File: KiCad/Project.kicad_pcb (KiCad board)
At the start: 2 copper layers, 0 parts

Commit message: Updated the schematics and started with the PCB
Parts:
- added C1, C2: 22pF, Capacitors_ThroughHole:C_Disc_D3_P2.5, F.Cu at (148.5, 105.0)
- added C3, C5: 0.1uF, Capacitors_ThroughHole:C_Disc_D3_P2.5, F.Cu at (148.5, 105.0)
- added C4, C6: 1uF, Capacitors_ThroughHole:C_Radial_D5_L6_P2.5, F.Cu at (148.5, 105.0)
- added D1, D11, D12, D13, D14, D15, D16, D2, D5, D6, D7, D8: LED, Wire_Connections_Bridges:WireConnection_1.50mmDrill, F.Cu at (148.5, 105.0)
- added D10, D3, D4, D9: IR_Recieve, Wire_Connections_Bridges:WireConnection_1.50mmDrill, F.Cu at (148.5, 105.0)
- added DS1: I2C_LCD16X2, Pin_Headers:Pin_Header_Straight_2x03_Pitch2.00mm, F.Cu at (148.5, 105.0)
- added IC1: ATMEGA328-P, Housings_DIP:DIP-28_W7.62mm, F.Cu at (146.1, 104.1)
- added IC2, IC3: ATTINY85-P, Housings_DIP:DIP-8_W7.62mm, F.Cu at (148.5, 105.0)
- added IC4: ATMEGA8-P, Housings_DIP:DIP-28_W7.62mm, F.Cu at (148.5, 105.0)
- added M1, M2: Motor, Wire_Connections_Bridges:WireConnection_1.50mmDrill, F.Cu at (148.5, 105.0)
- added P1: CONN_02X03, Pin_Headers:Pin_Header_Angled_2x03, F.Cu at (148.5, 105.0)
- added Q2, Q3, Q4: Q_NPN_BCE, TO_SOT_Packages_THT:TO-92_Inline_Narrow_Oval, F.Cu at (148.5, 105.0)
- added Q5: NPN, TO_SOT_Packages_THT:TO-92_Inline_Narrow_Oval, F.Cu at (148.5, 105.0)
- added R1: 1k, Resistors_ThroughHole:Resistor_Vertical_RM5mm, F.Cu at (148.5, 105.0)
- added R10, R11, R16, R17: 100, Resistors_ThroughHole:Resistor_Vertical_RM5mm, F.Cu at (148.5, 105.0)
- added R12, R13, R14, R15, R18, R19, R31, R37, R8, R9: 22, Resistors_ThroughHole:Resistor_Vertical_RM5mm, F.Cu at (148.5, 105.0)
- added R2: 10k, Resistors_ThroughHole:Resistor_Vertical_RM5mm, F.Cu at (148.5, 105.0)
- added R20, R21, R29, R30, R5: 1K, Resistors_ThroughHole:Resistor_Vertical_RM5mm, F.Cu at (148.5, 105.0)
- added R22, R6: 330, Resistors_ThroughHole:Resistor_Vertical_RM5mm, F.Cu at (148.5, 105.0)
- added R3: Photores, Wire_Connections_Bridges:WireConnection_1.50mmDrill, F.Cu at (148.5, 105.0)
- added R32, R33: 10, Resistors_ThroughHole:Resistor_Vertical_RM5mm, F.Cu at (148.5, 105.0)
- added R34, R35, R36: R, Resistors_ThroughHole:Resistor_Vertical_RM5mm, F.Cu at (148.5, 105.0)
- added R38, R39: 56, Resistors_ThroughHole:Resistor_Vertical_RM5mm, F.Cu at (148.5, 105.0)
- added R7: 470, Resistors_ThroughHole:Resistor_Vertical_RM5mm, F.Cu at (148.5, 105.0)
- added SW1: Reverse, Wire_Connections_Bridges:WireConnection_1.50mmDrill, F.Cu at (148.5, 105.0)
- added SW2: Start, Wire_Connections_Bridges:WireConnection_1.50mmDrill, F.Cu at (148.5, 105.0)
- added SW3: Lights, Wire_Connections_Bridges:WireConnection_1.50mmDrill, F.Cu at (148.5, 105.0)
- added SW4: SW_PUSH, Wire_Connections_Bridges:WireConnection_1.50mmDrill, F.Cu at (148.5, 105.0)
- added U1: BlueSmirf, Pin_Headers:Pin_Header_Straight_1x06, F.Cu at (148.5, 105.0)
- added U2, U3: LM317, TO_SOT_Packages_THT:TO-220_Neutral123_Vertical, F.Cu at (148.5, 105.0)
- added U5: Linkura, Wire_Connections_Bridges:WireConnection_1.50mmDrill, F.Cu at (148.5, 105.0)
- added U6: SN754410NE, Housings_DIP:DIP-16_W7.62mm_LongPads, F.Cu at (148.5, 105.0)
- added Y1: Crystal, Crystals:Crystal_HC52-U_Vertical, F.Cu at (148.5, 105.0)
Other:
- board outline added: 170.2 x 123.2 mm

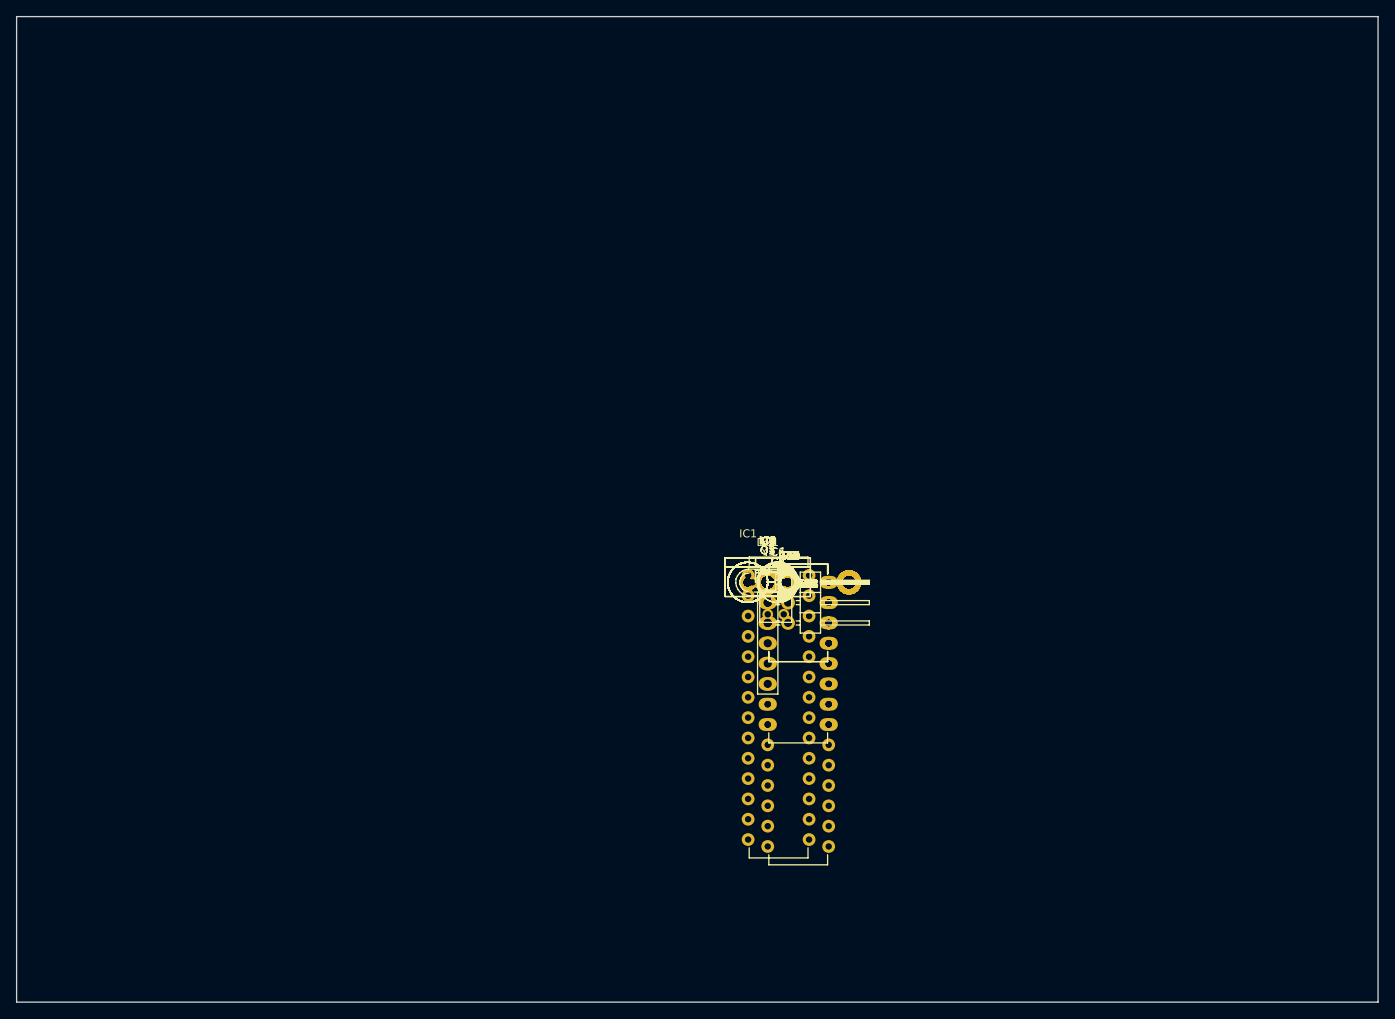
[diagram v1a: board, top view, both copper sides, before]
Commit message: Started with the PCB
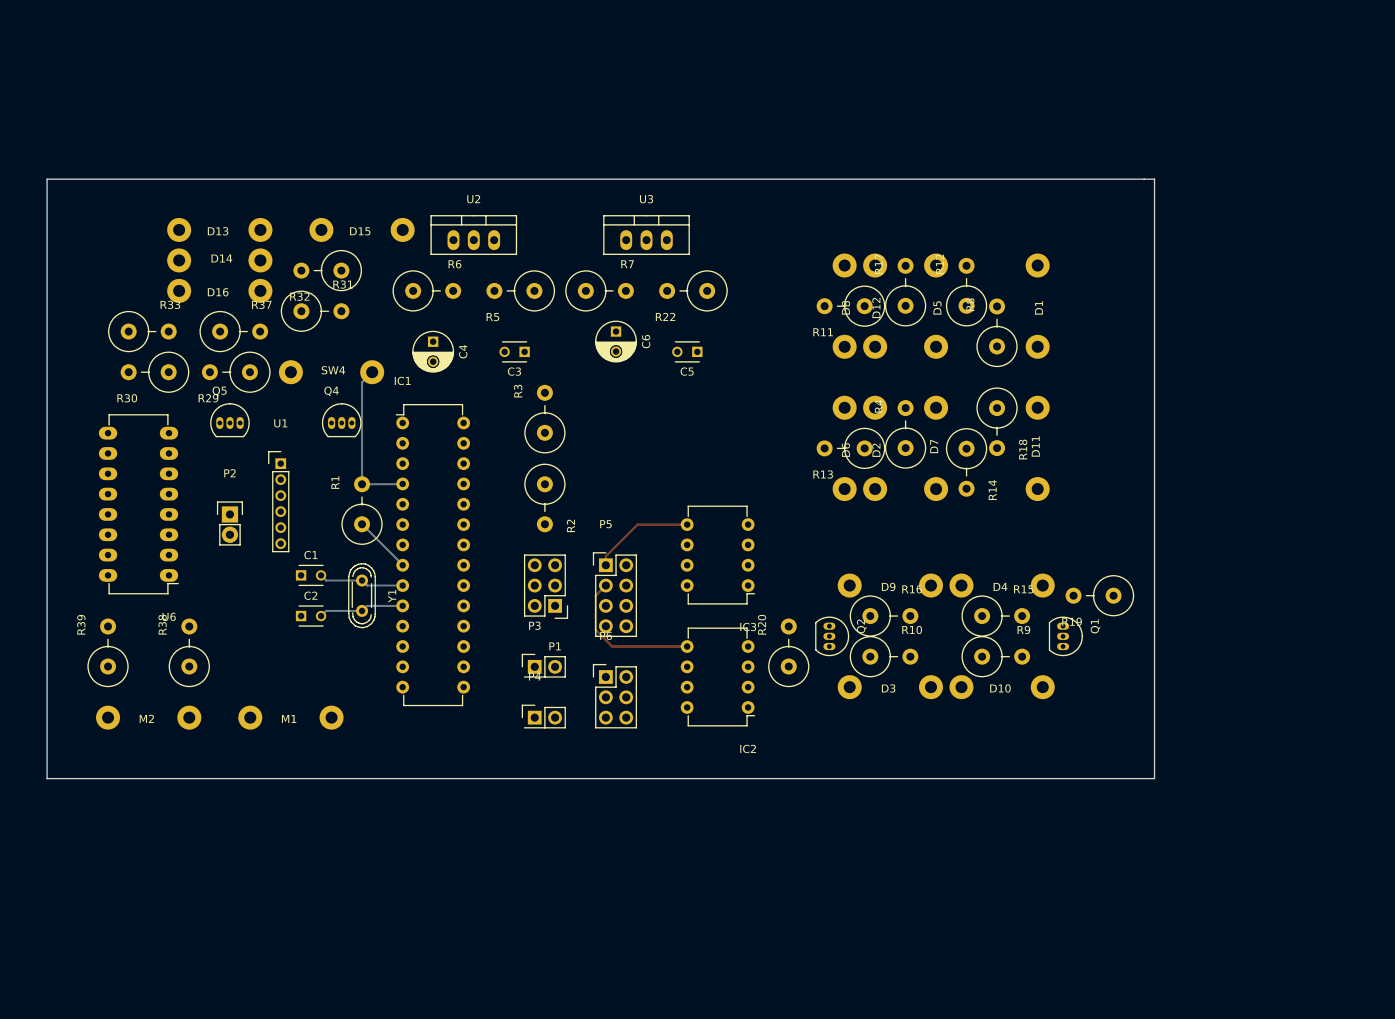
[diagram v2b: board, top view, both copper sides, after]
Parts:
- removed DS1: I2C_LCD16X2, Pin_Headers:Pin_Header_Straight_2x03_Pitch2.00mm
- removed IC4: ATMEGA8-P, Housings_DIP:DIP-28_W7.62mm
- removed Q3: Q_NPN_BCE, TO_SOT_Packages_THT:TO-92_Inline_Narrow_Oval
- removed R21: 1K, Resistors_ThroughHole:Resistor_Vertical_RM5mm
- removed R34, R35, R36: R, Resistors_ThroughHole:Resistor_Vertical_RM5mm
- removed SW1: Reverse, Wire_Connections_Bridges:WireConnection_1.50mmDrill
- removed SW2: Start, Wire_Connections_Bridges:WireConnection_1.50mmDrill
- removed SW3: Lights, Wire_Connections_Bridges:WireConnection_1.50mmDrill
- removed U5: Linkura, Wire_Connections_Bridges:WireConnection_1.50mmDrill
- added P2: CONN_01X02, Pin_Headers:Pin_Header_Straight_1x02, F.Cu at (81.3, 96.5)
- added P3: CONN_01X02, Pin_Headers:Pin_Header_Straight_2x01, F.Cu at (119.4, 115.6)
- added P4: CONN_01X02, Pin_Headers:Pin_Header_Straight_2x01, F.Cu at (119.4, 121.9)
- added P5: CONN_02X04, Pin_Headers:Pin_Header_Straight_2x04, F.Cu at (128.3, 102.9)
- added P6: CONN_02X03, Pin_Headers:Pin_Header_Straight_2x03, F.Cu at (128.3, 116.8)
- added Q1: Q_NPN_BCE, TO_SOT_Packages_THT:TO-92_Inline_Narrow_Oval, F.Cu at (185.4, 110.5)
- added R4: 22, Resistors_ThroughHole:Resistor_Vertical_RM5mm, F.Cu at (165.7, 85.7)
- P1: footprint Pin_Headers:Pin_Header_Angled_2x03 -> Pin_Headers:Pin_Header_Straight_2x03
- R11, R17: value 100 -> 22
- R15, R9: value 22 -> 100
- R19: value 22 -> 1K
- R3: footprint Wire_Connections_Bridges:WireConnection_1.50mmDrill -> Resistors_ThroughHole:Resistor_Vertical_RM5mm
- U1: footprint Pin_Headers:Pin_Header_Straight_1x06 -> Pin_Headers:Pin_Header_Straight_1x06_Pitch2.00mm
- moved D13 85.7 mm to (74.9, 61.0)
- moved M2 84.2 mm to (66.0, 121.9)
- moved R33 83.5 mm to (71.1, 73.7)
- moved R39 82.9 mm to (66.0, 113.0), turned to 90 degrees
- moved D16 82.1 mm to (74.9, 68.6)
- moved R30 81.7 mm to (71.1, 78.7), turned to 180 degrees
- moved D14 75.1 mm to (85.1, 64.8), turned to 180 degrees
- moved U6 74.8 mm to (73.7, 104.1), turned to 180 degrees
- moved R37 73.0 mm to (82.5, 73.7)
- moved R38 72.7 mm to (76.2, 113.0), turned to 90 degrees
- moved R29 72.2 mm to (81.3, 78.7), turned to 180 degrees
- moved Q5 71.3 mm to (80.0, 85.1)
- moved D15 71.1 mm to (92.7, 61.0)
- moved R32 68.1 mm to (92.7, 66.0), turned to 180 degrees
- moved M1 66.9 mm to (83.8, 121.9)
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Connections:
- IC2 pad 7: /IR/SCL -> Net-(IC2-Pad7)
- IC3 pad 1: Net-(IC3-Pad1) -> Net-(IC2-Pad1)
- IC3 pad 7: /IR/SCL -> Net-(IC2-Pad7)
- P1 pad 2: /IR/5V -> Net-(P1-Pad2)
- R11 pad 1: /IR/5V -> /IR/3V
- R11 pad 2: /IR/Signal -> Net-(D6-Pad2)
- R13 pad 2: Net-(D6-Pad2) -> Net-(D8-Pad2)
- R15 pad 1: /IR/3V -> /IR/5V
- R15 pad 2: Net-(D8-Pad2) -> /IR/Signal
- R17 pad 1: /IR/5V -> /IR/3V
- R17 pad 2: /IR/Signal -> Net-(D12-Pad2)
- R19 pad 1: /IR/3V -> Net-(IC2-Pad1)
- R19 pad 2: Net-(D12-Pad2) -> Net-(Q1-Pad1)
- R9 pad 1: /IR/3V -> /IR/5V
- R9 pad 2: Net-(D2-Pad2) -> /IR/Signal
- U1 pad 1: (no net) -> Net-(U1-Pad1)
- U1 pad 2: (no net) -> /IR/5V
- U1 pad 3: (no net) -> GND
- U1 pad 4: (no net) -> Net-(IC1-Pad2)
- U1 pad 5: (no net) -> Net-(IC1-Pad3)
- U1 pad 6: (no net) -> Net-(U1-Pad6)
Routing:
- net /IR/SDA: track 0.00 -> 31.3 mm
- net Net-(IC1-Pad4): track 0.00 -> 19.6 mm
- net Net-(C2-Pad2): track 0.00 -> 10.7 mm
- net Net-(C1-Pad2): track 0.00 -> 10.7 mm
- net GND: track 0.00 -> 7.22 mm
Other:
- board size 170.2 x 123.2 mm -> 138.4 x 74.9 mm
